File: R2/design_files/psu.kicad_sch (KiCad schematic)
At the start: 13 parts, among them U7 PUMH10,115, U8 LMR51430

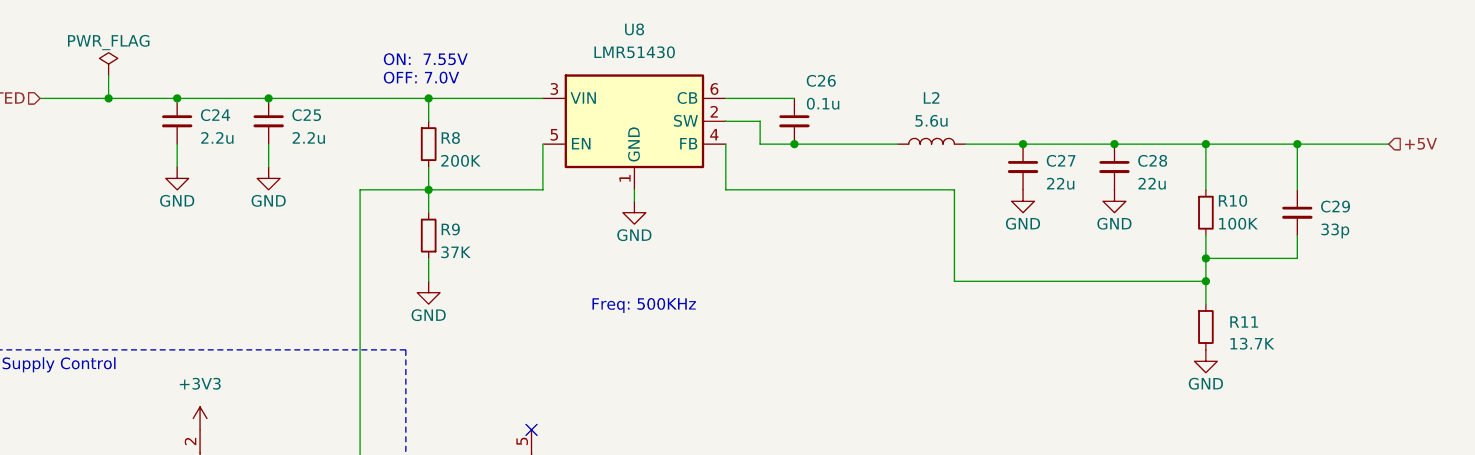
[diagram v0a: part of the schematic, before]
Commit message: Refactor code structure for improved readability and maintainability
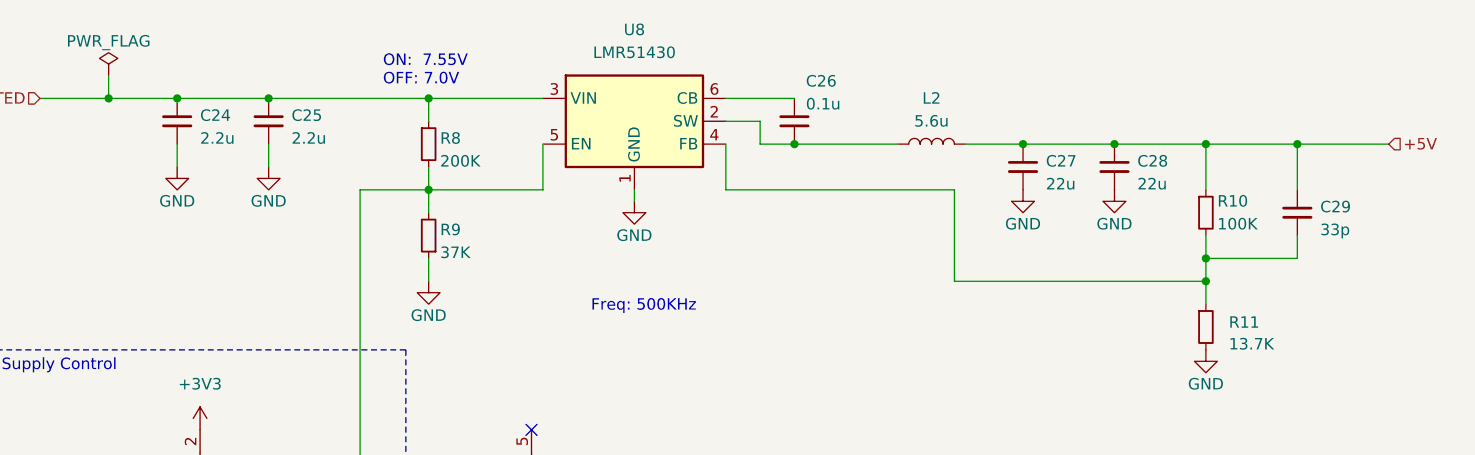
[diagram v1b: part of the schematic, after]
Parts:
- U7: symbol My Libraries:PUMH10,115 -> My_Libraries:PUMH10,115
